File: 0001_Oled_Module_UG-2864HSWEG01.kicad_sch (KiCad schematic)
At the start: 26 parts, among them SW1 SW_MEC_5E, SW2 SW_MEC_5E, SW3 SW_MEC_5E, SW4 SW_MEC_5E, SW5 SW_MEC_5E, SW6 SW_MEC_5E, U2 UG-2864HSWEG01

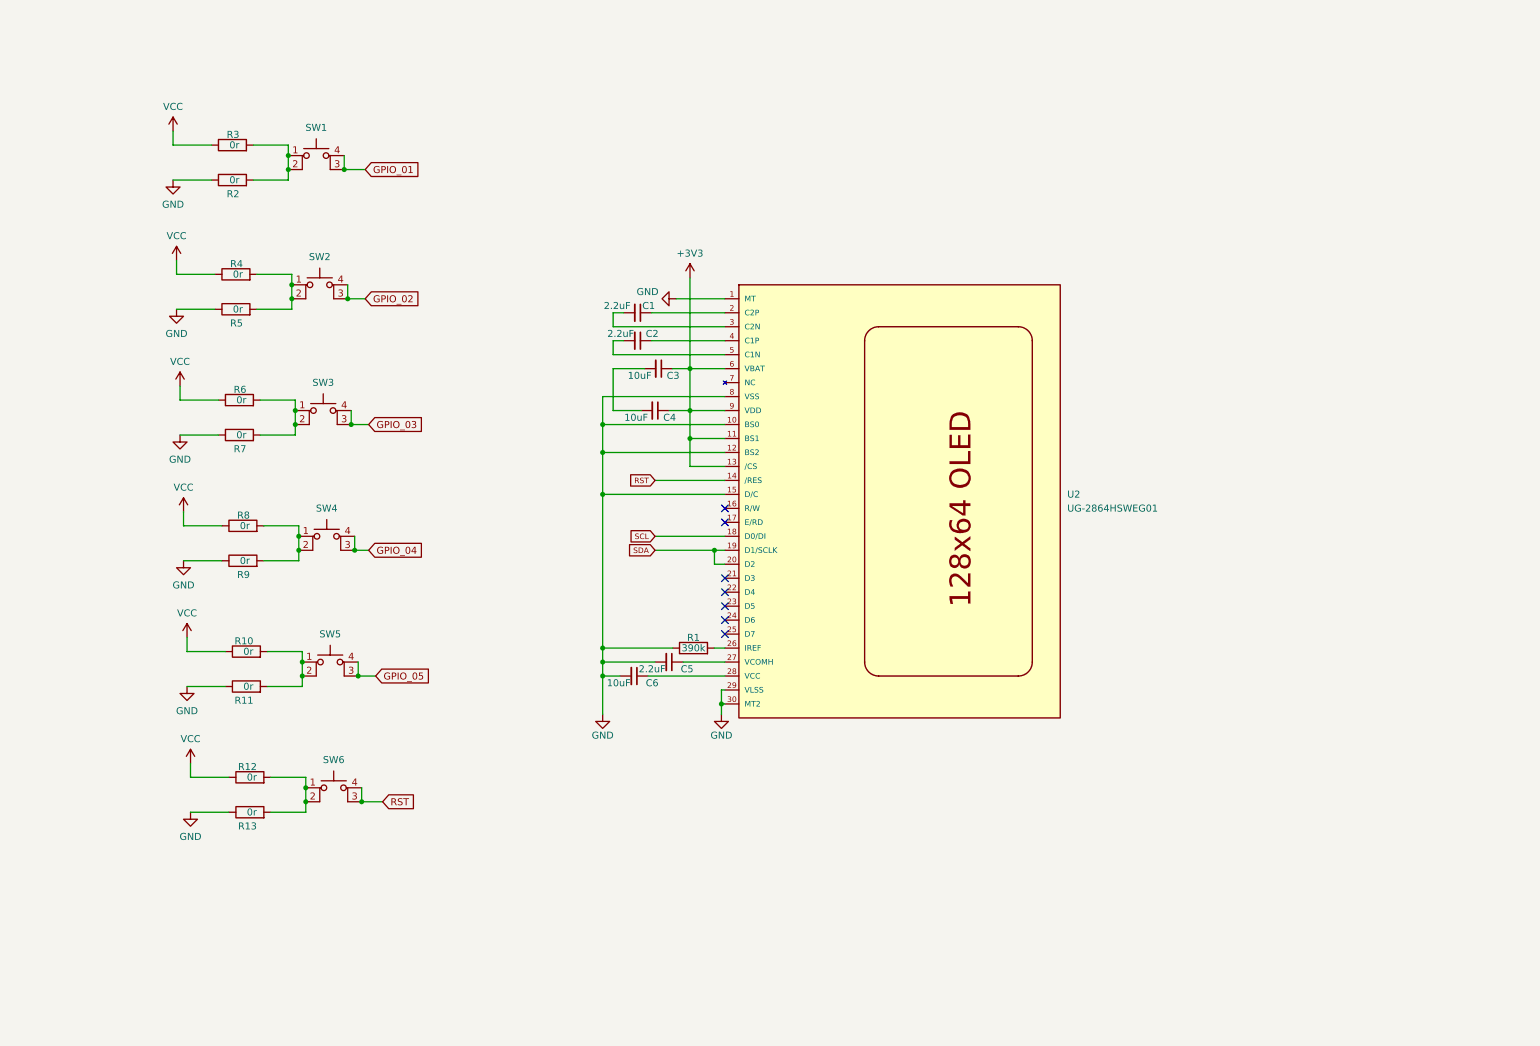
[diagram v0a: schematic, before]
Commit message: Add files via upload
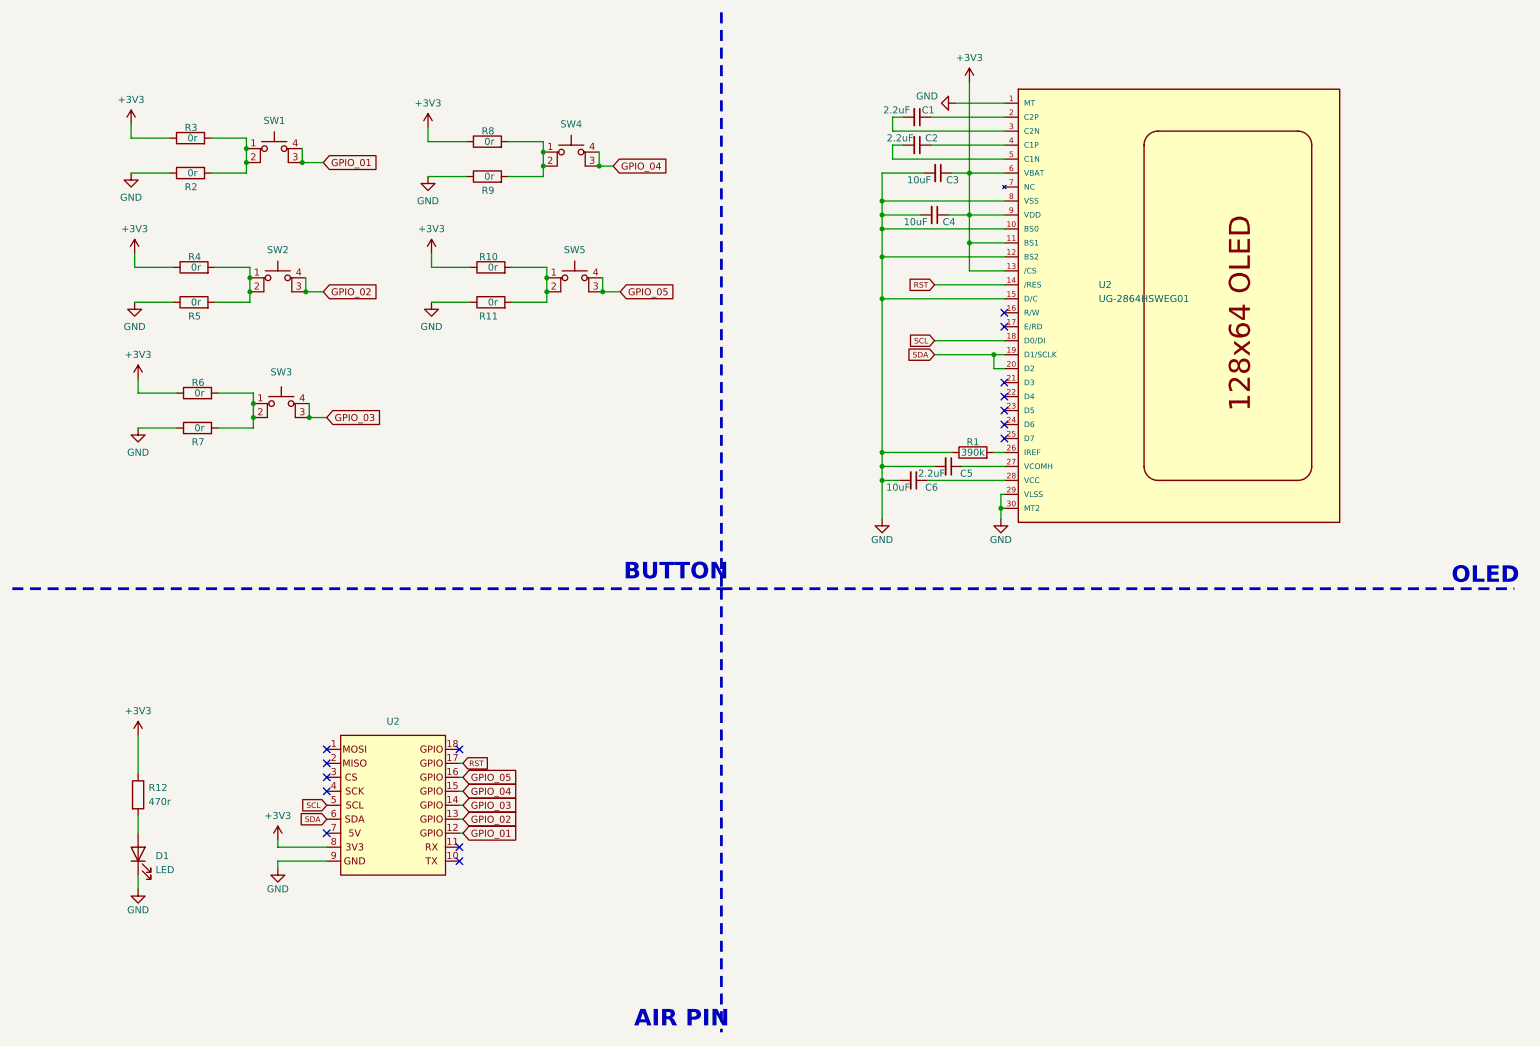
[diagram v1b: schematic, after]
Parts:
- removed R13: 0r, symbol Device:R
- removed SW6: SW_MEC_5E, button:button01, symbol Switch:SW_MEC_5E
- added D1: LED, LED_SMD:LED_0603_1608Metric, symbol Device:LED
- added U2: ~, Moduler_:pin_header_5-3, symbol moduler_pin:air
- C1, C2, C3, C4, C5, C6: footprint (none) -> Capacitor_SMD:C_0603_1608Metric
- R1, R10, R11, R2, R3, R4, R5, R6, R7, R8, R9: footprint (none) -> Resistor_SMD:R_0603_1608Metric
- R12: value 0r -> 470r; footprint (none) -> Resistor_SMD:R_0603_1608Metric
- SW1, SW2, SW3, SW4, SW5: footprint button:button01 -> oled_button:TS046665BK160SMT
- U2: footprint 1X30-0.7MM -> SSD1306:1X30-0.7MM
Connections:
- net VCC is gone; now on net +3V3: R10.1, R12.1, R3.1, R4.1, R6.1, R8.1
- net +3V3: now also U2.8
- net GND: now also C3.2, C4.2, D1.1 (K), U2.9
- net GPIO_01: now also U2.12
- net GPIO_02: now also U2.13
- net GPIO_03: now also U2.14
- net GPIO_04: now also U2.15
- net GPIO_05: now also U2.16
- net RST: now also U2.17
- net SCL: now also U2.5
- net SDA: now also U2.6
- net at R12.2: now also D1.2 (A)
- no-connect marks 7 -> 15
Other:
- note added: "AIR PIN"
- note added: "BUTTON"
- note added: "OLED"
- moved on the sheet: C1, C2, C3, C4, C5, C6, R1, R10, R11, R2, R3, R4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
